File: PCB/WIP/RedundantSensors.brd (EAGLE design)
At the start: 113 x 105.1 mm, 176 parts, among them J1 10118192-0001LF, J3 503182-1852, J4 JST-SH-4_SMT_V, U1 TPD4F003DQDR, U10 LIS3MDLTR, U2 BMI088, U3 BMI088, U4 BMI088, U5 STM32H743ZIT6, U6 LIS3MDLTR, U7 LIS3MDLTR, X1 LiDAR, X2 Telemetry, X3 RC, Y2 8MHz

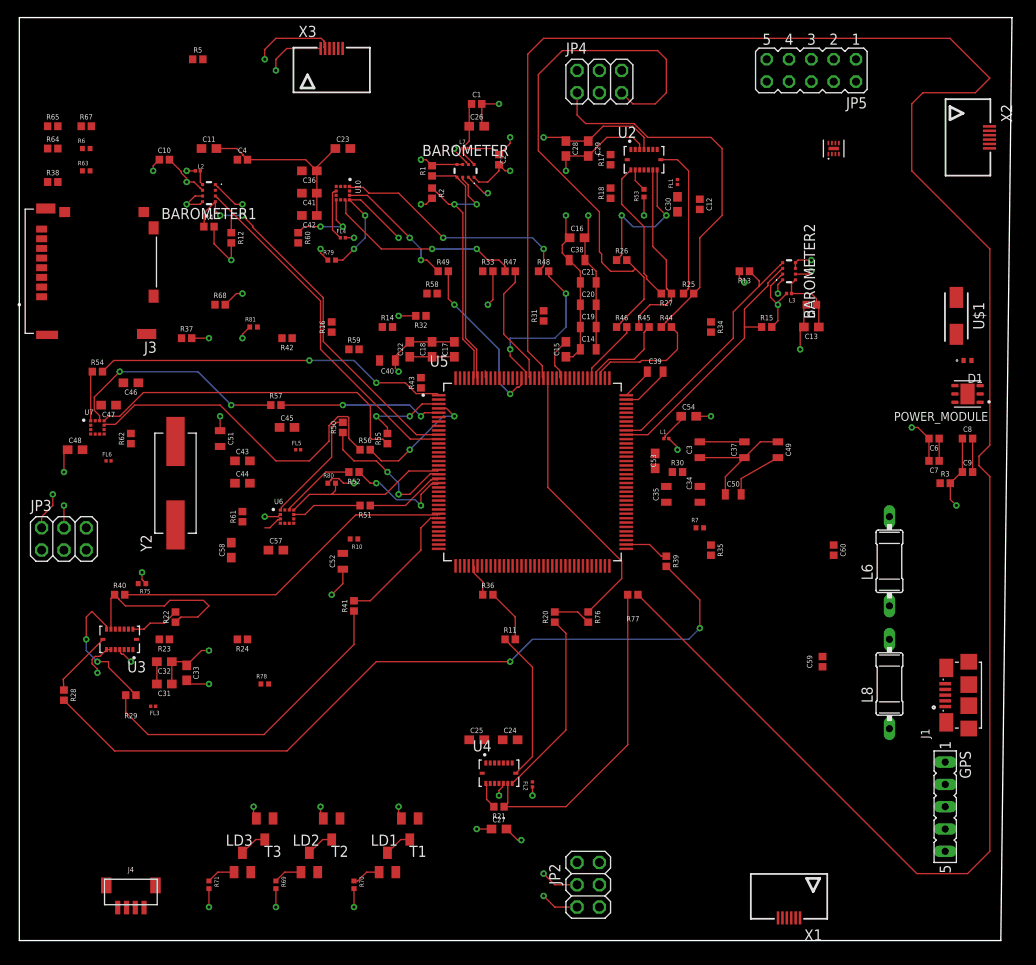
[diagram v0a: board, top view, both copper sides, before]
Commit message: edison autoroute
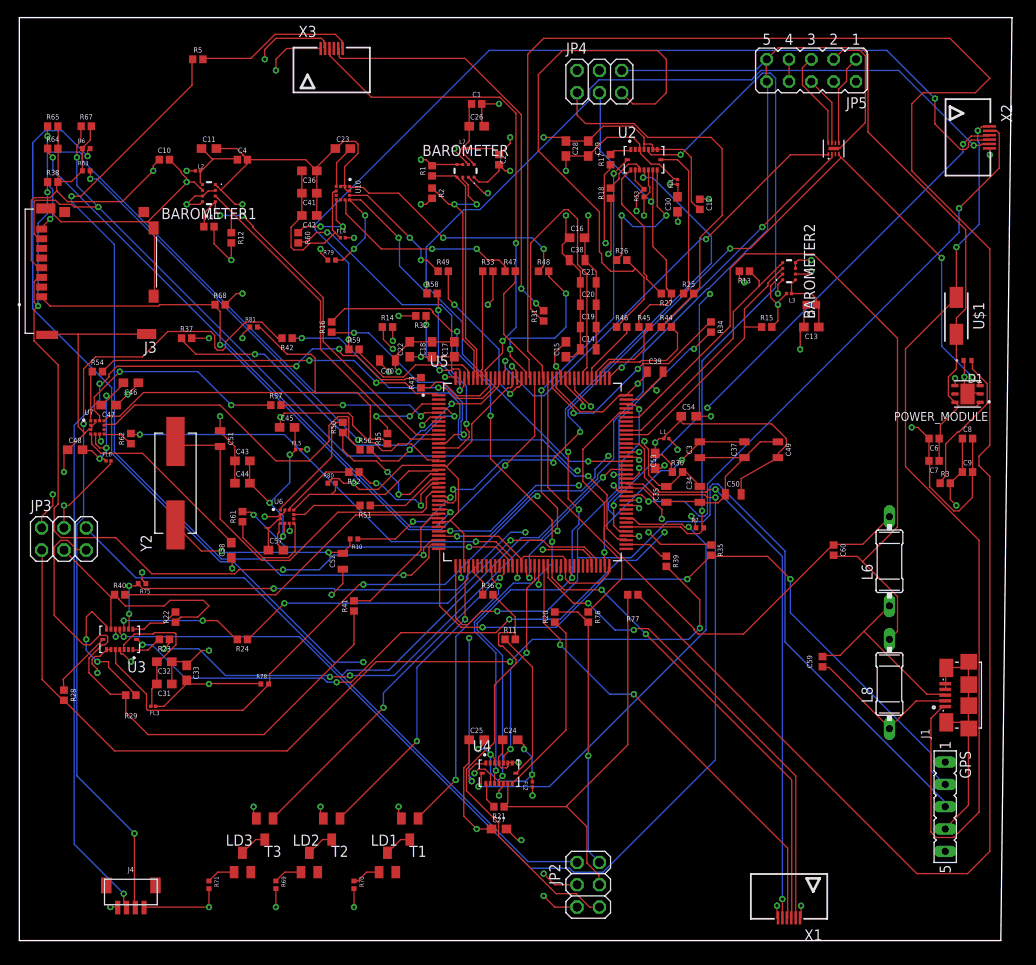
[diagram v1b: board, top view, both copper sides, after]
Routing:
- net 5V: track 2.54 -> 251.3 mm
- net GND: track 167.4 -> 385.0 mm, vias 28 -> 46
- net 3V3: track 125.1 -> 287.1 mm, vias 33 -> 47
- net USART2_RX: track 0.00 -> 125.9 mm, vias 0 -> 2
- net DRDY2_GYRO3: track 0.00 -> 125.5 mm, vias 0 -> 2
- net 5V_IN: track 0.00 -> 108.2 mm, vias 0 -> 2
- net UART8_RX: track 0.00 -> 107.9 mm, vias 0 -> 2
- net CSB_ACCEL4: track 0.00 -> 107.8 mm, vias 0 -> 3
- net SDMCC_D1: track 0.00 -> 104.2 mm, vias 0 -> 4
- net UART5_TX: track 0.00 -> 103.6 mm, vias 0 -> 4
- net SDMCC_D0: track 0.00 -> 100.9 mm, vias 0 -> 3
- net NRST: track 0.00 -> 100.3 mm, vias 0 -> 6
- net CSB_GYRO1: track 0.00 -> 99.8 mm, vias 0 -> 4
- net N$20: track 0.00 -> 98.0 mm, vias 0 -> 2
- net SDMCC_CMD: track 0.00 -> 93.5 mm, vias 0 -> 4
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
